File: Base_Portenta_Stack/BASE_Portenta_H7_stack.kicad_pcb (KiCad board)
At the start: 2 copper layers, 79.8 x 26.6 mm, 19 parts, among them J4 PinHeader_1x04_P2.00mm_Vertic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

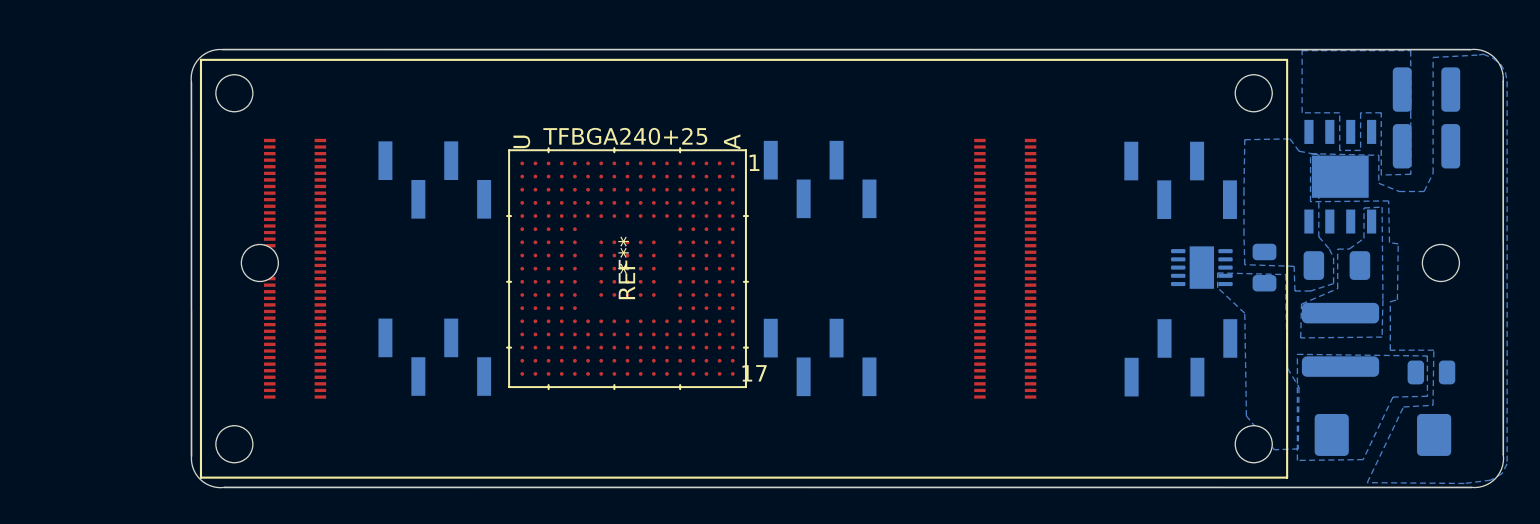
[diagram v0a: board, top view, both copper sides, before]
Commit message: Update BASE_Portenta_H7_stack.kicad_pcb
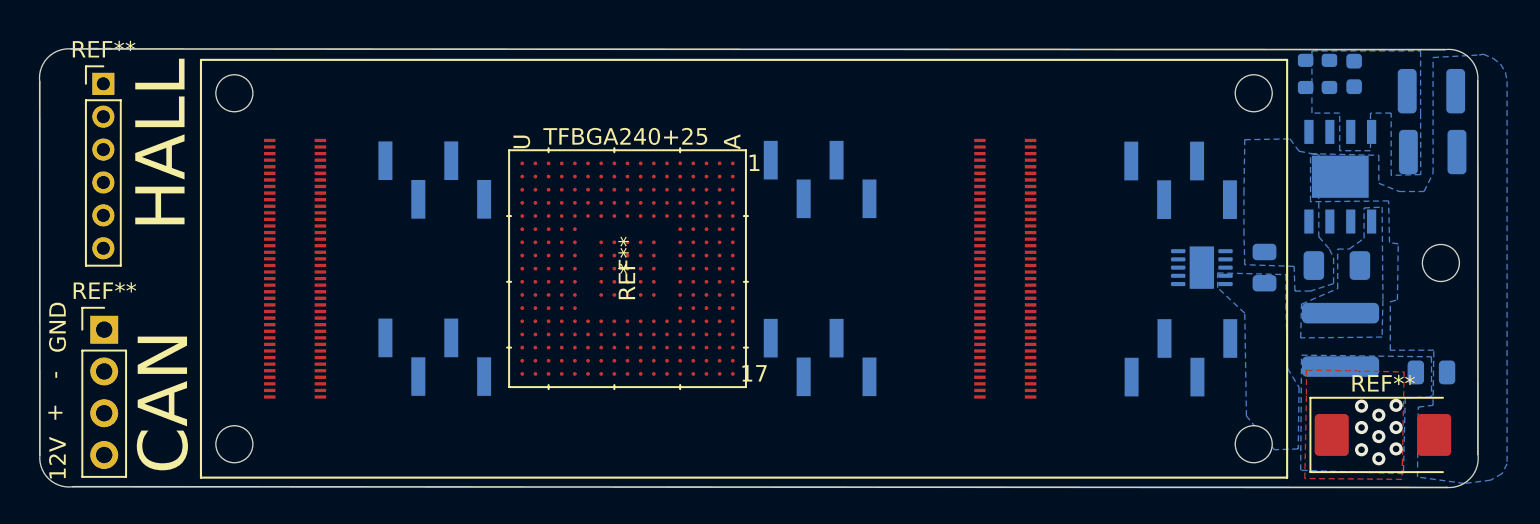
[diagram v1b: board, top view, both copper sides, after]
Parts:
- removed the REF** at (110.4, 93.4)
- added REF**: PinHeader_1x04_P2.54mm_Vertical, Connector_PinHeader_2.54mm:PinHeader_1x04_P2.54mm_Vertical, F.Cu at (100.9, 97.5)
- added REF**: R_0603_1608Metric, Resistor_SMD:R_0603_1608Metric, B.Cu at (173.9, 82.0)
- added REF**: R_0603_1608Metric, Resistor_SMD:R_0603_1608Metric, B.Cu at (175.4, 82.0)
- added REF**: C_0603_1608Metric, Capacitor_SMD:C_0603_1608Metric, B.Cu at (176.9, 82.0)
- added REF**: PinHeader_1x06_P2.00mm_Vertical, Connector_PinHeader_2.00mm:PinHeader_1x06_P2.00mm_Vertical, F.Cu at (100.8, 82.5)
- REF**: moved to F.Cu
- U1: renamed from REF**; value MODULE_ABX00042 -> ABX00042
- moved REF** 0.51 mm to (181.7, 86.7)
- moved REF** 0.32 mm to (181.6, 83.0)
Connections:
- U1 pad J1_1: (no net) -> unconnected-(U1-PadJ1_1)
- U1 pad J1_10: (no net) -> unconnected-(U1-PadJ1_10)
- U1 pad J1_11: (no net) -> unconnected-(U1-PadJ1_11)
- U1 pad J1_12: (no net) -> unconnected-(U1-PadJ1_12)
- U1 pad J1_13: (no net) -> unconnected-(U1-PadJ1_13)
- U1 pad J1_14: (no net) -> unconnected-(U1-PadJ1_14)
- U1 pad J1_15: (no net) -> unconnected-(U1-PadJ1_15)
- U1 pad J1_16: (no net) -> unconnected-(U1-PadJ1_16)
- U1 pad J1_17: (no net) -> unconnected-(U1-PadJ1_17)
- U1 pad J1_18: (no net) -> unconnected-(U1-PadJ1_18)
- U1 pad J1_19: (no net) -> unconnected-(U1-PadJ1_19)
- U1 pad J1_2: (no net) -> unconnected-(U1-PadJ1_2)
- U1 pad J1_20: (no net) -> unconnected-(U1-PadJ1_20)
- U1 pad J1_21: (no net) -> Net-(U1-PadJ1_21)
- U1 pad J1_22: (no net) -> Net-(U1-PadJ1_22)
- U1 pad J1_23: (no net) -> unconnected-(U1-PadJ1_23)
- U1 pad J1_24: (no net) -> unconnected-(U1-PadJ1_24)
- U1 pad J1_25: (no net) -> unconnected-(U1-PadJ1_25)
- U1 pad J1_26: (no net) -> unconnected-(U1-PadJ1_26)
- U1 pad J1_27: (no net) -> unconnected-(U1-PadJ1_27)
- U1 pad J1_28: (no net) -> unconnected-(U1-PadJ1_28)
- U1 pad J1_29: (no net) -> unconnected-(U1-PadJ1_29)
- U1 pad J1_3: (no net) -> unconnected-(U1-PadJ1_3)
- U1 pad J1_30: (no net) -> unconnected-(U1-PadJ1_30)
- U1 pad J1_31: (no net) -> Net-(U1-PadJ1_22)
- U1 pad J1_32: (no net) -> Net-(U1-PadJ1_21)
- U1 pad J1_33: (no net) -> unconnected-(U1-PadJ1_33)
- U1 pad J1_34: (no net) -> unconnected-(U1-PadJ1_34)
- U1 pad J1_35: (no net) -> unconnected-(U1-PadJ1_35)
- U1 pad J1_36: (no net) -> unconnected-(U1-PadJ1_36)
- U1 pad J1_37: (no net) -> unconnected-(U1-PadJ1_37)
- U1 pad J1_38: (no net) -> unconnected-(U1-PadJ1_38)
- U1 pad J1_39: (no net) -> unconnected-(U1-PadJ1_39)
- U1 pad J1_4: (no net) -> unconnected-(U1-PadJ1_4)
- U1 pad J1_40: (no net) -> unconnected-(U1-PadJ1_40)
- U1 pad J1_41: (no net) -> Net-(U1-PadJ1_21)
- U1 pad J1_42: (no net) -> Net-(U1-PadJ1_22)
- U1 pad J1_43: (no net) -> unconnected-(U1-PadJ1_43)
- U1 pad J1_44: (no net) -> unconnected-(U1-PadJ1_44)
- U1 pad J1_45: (no net) -> unconnected-(U1-PadJ1_45)
- U1 pad J1_46: (no net) -> unconnected-(U1-PadJ1_46)
- U1 pad J1_47: (no net) -> Net-(U1-PadJ1_22)
- U1 pad J1_48: (no net) -> Net-(U1-PadJ1_21)
- U1 pad J1_49: (no net) -> unconnected-(U1-PadJ1_49)
- U1 pad J1_5: (no net) -> unconnected-(U1-PadJ1_5)
- U1 pad J1_50: (no net) -> unconnected-(U1-PadJ1_50)
- U1 pad J1_51: (no net) -> unconnected-(U1-PadJ1_51)
- U1 pad J1_52: (no net) -> unconnected-(U1-PadJ1_52)
- U1 pad J1_53: (no net) -> Net-(U1-PadJ1_53)
- U1 pad J1_54: (no net) -> Net-(U1-PadJ1_22)
- U1 pad J1_55: (no net) -> unconnected-(U1-PadJ1_55)
- U1 pad J1_56: (no net) -> unconnected-(U1-PadJ1_56)
- U1 pad J1_57: (no net) -> unconnected-(U1-PadJ1_57)
- U1 pad J1_58: (no net) -> unconnected-(U1-PadJ1_58)
- U1 pad J1_59: (no net) -> unconnected-(U1-PadJ1_59)
- U1 pad J1_6: (no net) -> unconnected-(U1-PadJ1_6)
- U1 pad J1_60: (no net) -> unconnected-(U1-PadJ1_60)
- U1 pad J1_61: (no net) -> unconnected-(U1-PadJ1_61)
- U1 pad J1_62: (no net) -> unconnected-(U1-PadJ1_62)
- U1 pad J1_63: (no net) -> unconnected-(U1-PadJ1_63)
- U1 pad J1_64: (no net) -> Net-(U1-PadJ1_53)
- U1 pad J1_65: (no net) -> unconnected-(U1-PadJ1_65)
- U1 pad J1_66: (no net) -> unconnected-(U1-PadJ1_66)
- U1 pad J1_67: (no net) -> unconnected-(U1-PadJ1_67)
- U1 pad J1_68: (no net) -> unconnected-(U1-PadJ1_68)
- U1 pad J1_69: (no net) -> unconnected-(U1-PadJ1_69)
- U1 pad J1_7: (no net) -> unconnected-(U1-PadJ1_7)
- U1 pad J1_70: (no net) -> unconnected-(U1-PadJ1_70)
- U1 pad J1_71: (no net) -> unconnected-(U1-PadJ1_71)
- U1 pad J1_72: (no net) -> unconnected-(U1-PadJ1_72)
- U1 pad J1_73: (no net) -> unconnected-(U1-PadJ1_73)
- U1 pad J1_74: (no net) -> unconnected-(U1-PadJ1_74)
- U1 pad J1_75: (no net) -> unconnected-(U1-PadJ1_75)
- U1 pad J1_76: (no net) -> unconnected-(U1-PadJ1_76)
- U1 pad J1_77: (no net) -> unconnected-(U1-PadJ1_77)
- U1 pad J1_78: (no net) -> unconnected-(U1-PadJ1_78)
- U1 pad J1_79: (no net) -> unconnected-(U1-PadJ1_79)
- U1 pad J1_8: (no net) -> unconnected-(U1-PadJ1_8)
- U1 pad J1_80: (no net) -> unconnected-(U1-PadJ1_80)
- U1 pad J1_9: (no net) -> unconnected-(U1-PadJ1_9)
- U1 pad J2_1: (no net) -> unconnected-(U1-PadJ2_1)
- U1 pad J2_10: (no net) -> unconnected-(U1-PadJ2_10)
- U1 pad J2_11: (no net) -> unconnected-(U1-PadJ2_11)
- U1 pad J2_12: (no net) -> unconnected-(U1-PadJ2_12)
- U1 pad J2_13: (no net) -> unconnected-(U1-PadJ2_13)
- U1 pad J2_14: (no net) -> unconnected-(U1-PadJ2_14)
- U1 pad J2_15: (no net) -> unconnected-(U1-PadJ2_15)
- U1 pad J2_16: (no net) -> unconnected-(U1-PadJ2_16)
- U1 pad J2_17: (no net) -> unconnected-(U1-PadJ2_17)
- U1 pad J2_18: (no net) -> unconnected-(U1-PadJ2_18)
- U1 pad J2_19: (no net) -> unconnected-(U1-PadJ2_19)
- U1 pad J2_2: (no net) -> unconnected-(U1-PadJ2_2)
- U1 pad J2_20: (no net) -> unconnected-(U1-PadJ2_20)
- U1 pad J2_21: (no net) -> unconnected-(U1-PadJ2_21)
- U1 pad J2_22: (no net) -> unconnected-(U1-PadJ2_22)
- U1 pad J2_23: (no net) -> Net-(U1-PadJ2_23)
- U1 pad J2_24: (no net) -> Net-(U1-PadJ2_24)
- U1 pad J2_25: (no net) -> unconnected-(U1-PadJ2_25)
- U1 pad J2_26: (no net) -> unconnected-(U1-PadJ2_26)
- U1 pad J2_27: (no net) -> unconnected-(U1-PadJ2_27)
- U1 pad J2_28: (no net) -> unconnected-(U1-PadJ2_28)
- U1 pad J2_29: (no net) -> unconnected-(U1-PadJ2_29)
- U1 pad J2_3: (no net) -> unconnected-(U1-PadJ2_3)
- U1 pad J2_30: (no net) -> unconnected-(U1-PadJ2_30)
- U1 pad J2_31: (no net) -> unconnected-(U1-PadJ2_31)
- U1 pad J2_32: (no net) -> unconnected-(U1-PadJ2_32)
- U1 pad J2_33: (no net) -> Net-(U1-PadJ2_24)
- U1 pad J2_34: (no net) -> unconnected-(U1-PadJ2_34)
- U1 pad J2_35: (no net) -> unconnected-(U1-PadJ2_35)
- U1 pad J2_36: (no net) -> unconnected-(U1-PadJ2_36)
- U1 pad J2_37: (no net) -> unconnected-(U1-PadJ2_37)
- U1 pad J2_38: (no net) -> unconnected-(U1-PadJ2_38)
- U1 pad J2_39: (no net) -> unconnected-(U1-PadJ2_39)
- U1 pad J2_4: (no net) -> unconnected-(U1-PadJ2_4)
- U1 pad J2_40: (no net) -> unconnected-(U1-PadJ2_40)
- U1 pad J2_41: (no net) -> unconnected-(U1-PadJ2_41)
- U1 pad J2_42: (no net) -> unconnected-(U1-PadJ2_42)
- U1 pad J2_43: (no net) -> Net-(U1-PadJ2_23)
- U1 pad J2_44: (no net) -> Net-(U1-PadJ2_24)
- U1 pad J2_45: (no net) -> unconnected-(U1-PadJ2_45)
- U1 pad J2_46: (no net) -> unconnected-(U1-PadJ2_46)
- U1 pad J2_47: (no net) -> unconnected-(U1-PadJ2_47)
- U1 pad J2_48: (no net) -> unconnected-(U1-PadJ2_48)
- U1 pad J2_49: (no net) -> unconnected-(U1-PadJ2_49)
- U1 pad J2_5: (no net) -> unconnected-(U1-PadJ2_5)
- U1 pad J2_50: (no net) -> unconnected-(U1-PadJ2_50)
- U1 pad J2_51: (no net) -> unconnected-(U1-PadJ2_51)
- U1 pad J2_52: (no net) -> unconnected-(U1-PadJ2_52)
- U1 pad J2_53: (no net) -> unconnected-(U1-PadJ2_53)
- U1 pad J2_54: (no net) -> unconnected-(U1-PadJ2_54)
- U1 pad J2_55: (no net) -> unconnected-(U1-PadJ2_55)
- U1 pad J2_56: (no net) -> unconnected-(U1-PadJ2_56)
- U1 pad J2_57: (no net) -> Net-(U1-PadJ2_24)
- U1 pad J2_58: (no net) -> unconnected-(U1-PadJ2_58)
- U1 pad J2_59: (no net) -> unconnected-(U1-PadJ2_59)
- U1 pad J2_6: (no net) -> unconnected-(U1-PadJ2_6)
- U1 pad J2_60: (no net) -> unconnected-(U1-PadJ2_60)
- U1 pad J2_61: (no net) -> unconnected-(U1-PadJ2_61)
- U1 pad J2_62: (no net) -> unconnected-(U1-PadJ2_62)
- U1 pad J2_63: (no net) -> unconnected-(U1-PadJ2_63)
- U1 pad J2_64: (no net) -> unconnected-(U1-PadJ2_64)
- U1 pad J2_65: (no net) -> unconnected-(U1-PadJ2_65)
- U1 pad J2_66: (no net) -> unconnected-(U1-PadJ2_66)
- U1 pad J2_67: (no net) -> unconnected-(U1-PadJ2_67)
- U1 pad J2_68: (no net) -> unconnected-(U1-PadJ2_68)
- U1 pad J2_69: (no net) -> Net-(U1-PadJ2_23)
- U1 pad J2_7: (no net) -> unconnected-(U1-PadJ2_7)
- U1 pad J2_70: (no net) -> Net-(U1-PadJ2_24)
- U1 pad J2_71: (no net) -> unconnected-(U1-PadJ2_71)
- U1 pad J2_72: (no net) -> unconnected-(U1-PadJ2_72)
- U1 pad J2_73: (no net) -> unconnected-(U1-PadJ2_73)
- U1 pad J2_74: (no net) -> unconnected-(U1-PadJ2_74)
- U1 pad J2_75: (no net) -> unconnected-(U1-PadJ2_75)
- U1 pad J2_76: (no net) -> unconnected-(U1-PadJ2_76)
- U1 pad J2_77: (no net) -> unconnected-(U1-PadJ2_77)
- U1 pad J2_78: (no net) -> unconnected-(U1-PadJ2_78)
- U1 pad J2_79: (no net) -> unconnected-(U1-PadJ2_79)
- U1 pad J2_8: (no net) -> unconnected-(U1-PadJ2_8)
- U1 pad J2_80: (no net) -> unconnected-(U1-PadJ2_80)
- U1 pad J2_9: (no net) -> unconnected-(U1-PadJ2_9)
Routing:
- net SWT_OUT_12V: vias 0 -> 9
- added copper zone on F.Cu, net SWT_OUT_12V
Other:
- board size 79.8 x 26.6 mm -> 87.5 x 26.7 mm
- board text added: "+"
- board text added: "-"
- board text added: "12V"
- board text added: "CAN"
- board text added: "GND"
- board text added: "HALL"

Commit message: Log
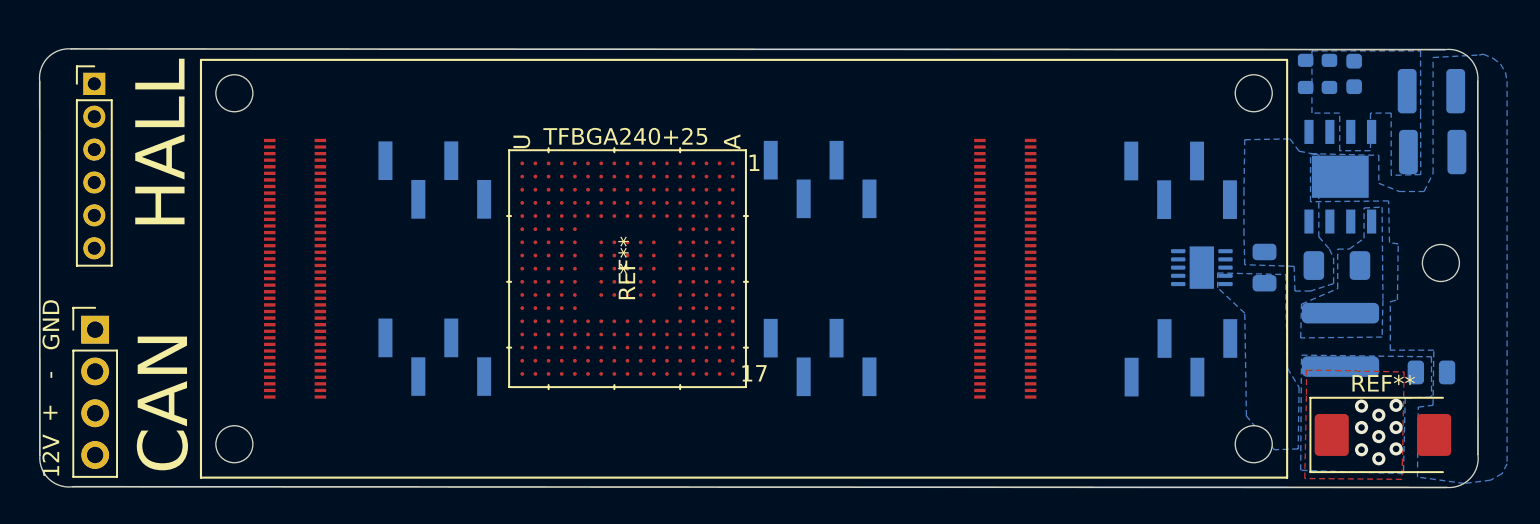
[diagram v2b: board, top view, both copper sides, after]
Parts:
- moved REF** 0.55 mm to (100.3, 97.5)
- moved REF** 0.55 mm to (100.3, 82.5)
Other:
- outline, holes or cut-outs redrawn
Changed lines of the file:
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@@
   (net 157 "unconnected-(U1-PadJ2_80)")
   (footprint "Connector_PinHeader_2.54mm:PinHeader_1x04_P2.54mm_Vertical" (layer "F.Cu")
-    (at 100.9 97.5)
+    (at 100.35 97.5)
     (descr "Through hole straight pin header, 1x04, 2.54mm pitch, single row")
     (tags "Through hole pin header THT 1x04 2.54mm single row")
     (attr through_hole)
-    (fp_text reference "REF**" (at 0 -2.33) (layer "F.SilkS")
+    (fp_text reference "REF**" (at 0 -2.33) (layer "F.SilkS") hide
       (effects (font (size 1 1) (thickness 0.15)))
     )
-    (fp_text value "PinHeader_1x04_P2.54mm_Vertical" (at 0 9.95) (layer "F.Fab")
+    (fp_text value "PinHeader_1x04_P2.54mm_Vertical" (at 0 9.95) (layer "F.Fab") hide
       (effects (font (size 1 1) (thickness 0.15)))
     )
-    (fp_text user "${REFERENCE}" (at 0 3.81 90) (layer "F.Fab")
+    (fp_text user "${REFERENCE}" (at 0 3.81 90) (layer "F.Fab") hide
       (effects (font (size 1 1) (thickness 0.15)))
     )
@@
     (pad "4" thru_hole oval (at 0 7.62) (size 1.7 1.7) (drill 1) (layers *.Cu *.Mask)
       (net 11 "SWT_OUT_12V"))
-    (model "${KICAD6_3DMODEL_DIR}/Connector_PinHeader_2.54mm.3dshapes/PinHeader_1x04_P2.54mm_Vertical.wrl"
+    (model "${KICAD6_3DMODEL_DIR}/Connector_PinHeader_2.54mm.3dshapes/PinHeader_1x04_P2.54mm_Vertical.wrl" hide
       (offset (xyz 0 0 0))
       (scale (xyz 1 1 1))
@@
   )
   (footprint "Connector_PinHeader_2.00mm:PinHeader_1x06_P2.00mm_Vertical" (layer "F.Cu")
-    (at 100.85 82.55)
+    (at 100.3 82.55)
     (descr "Through hole straight pin header, 1x06, 2.00mm pitch, single row")
     (tags "Through hole pin header THT 1x06 2.00mm single row")
     (attr through_hole)
-    (fp_text reference "REF**" (at 0 -2.06) (layer "F.SilkS")
+    (fp_text reference "REF**" (at 0 -2.06) (layer "F.SilkS") hide
       (effects (font (size 1 1) (thickness 0.15)))
     )
-    (fp_text value "PinHeader_1x06_P2.00mm_Vertical" (at 0 12.06) (layer "F.Fab")
+    (fp_text value "PinHeader_1x06_P2.00mm_Vertical" (at 0 12.06) (layer "F.Fab") hide
       (effects (font (size 1 1) (thickness 0.15)))
     )
-    (fp_text user "${REFERENCE}" (at 0 5 90) (layer "F.Fab")
+    (fp_text user "${REFERENCE}" (at 0 5 90) (layer "F.Fab") hide
       (effects (font (size 1 1) (thickness 0.15)))
     )
@@
     (pad "5" thru_hole oval (at 0 8) (size 1.35 1.35) (drill 0.8) (layers *.Cu *.Mask))
     (pad "6" thru_hole oval (at 0 10) (size 1.35 1.35) (drill 0.8) (layers *.Cu *.Mask))
-    (model "${KICAD6_3DMODEL_DIR}/Connector_PinHeader_2.00mm.3dshapes/PinHeader_1x06_P2.00mm_Vertical.wrl"
+    (model "${KICAD6_3DMODEL_DIR}/Connector_PinHeader_2.00mm.3dshapes/PinHeader_1x06_P2.00mm_Vertical.wrl" hide
       (offset (xyz 0 0 0))
       (scale (xyz 1 1 1))
@@
   )
   (gr_arc (start 182.41 80.472791) (mid 183.879437 80.95) (end 184.42 82.392791) (layer "Edge.Cuts") (width 0.05))
-  (gr_line (start 182.557209 107.093354) (end 99 107.05) (layer "Edge.Cuts") (width 0.1))
+  (gr_line (start 182.507209 107.093354) (end 99 107.05) (layer "Edge.Cuts") (width 0.1))
   (gr_arc (start 184.427209 105.083354) (mid 183.95 106.552791) (end 182.507209 107.093354) (layer "Edge.Cuts") (width 0.05))
   (gr_arc (start 99 107.05) (mid 97.530563 106.572791) (end 96.99 105.13) (layer "Edge.Cuts") (width 0.05))
@@
   (gr_line (start 96.99 105.13) (end 96.982791 82.439437) (layer "Edge.Cuts") (width 0.1))
   (gr_line (start 184.42 82.392791) (end 184.427209 105.083354) (layer "Edge.Cuts") (width 0.1))
-  (gr_text "+" (at 97.9 102.55 90) (layer "F.SilkS")
+  (gr_text "+" (at 97.6 102.55 90) (layer "F.SilkS")
     (effects (font (size 1 1) (thickness 0.2)))
   )
-  (gr_text "-" (at 97.9 100.25 90) (layer "F.SilkS")
+  (gr_text "-" (at 97.6 100.25 90) (layer "F.SilkS")
     (effects (font (size 1 1) (thickness 0.2)))
   )
@@
     (effects (font (size 3 3) (thickness 0.75)))
   )
-  (gr_text "GND" (at 98.1 97.35 90) (layer "F.SilkS")
+  (gr_text "GND" (at 97.7 97.2 90) (layer "F.SilkS")
     (effects (font (size 1 1) (thickness 0.2)))
   )
@@
     (effects (font (size 3 3) (thickness 0.75)))
   )
-  (gr_text "12V" (at 98.1 105.35 90) (layer "F.SilkS")
+  (gr_text "12V" (at 97.7 105.2 90) (layer "F.SilkS")
     (effects (font (size 1 1) (thickness 0.2)))
   )
